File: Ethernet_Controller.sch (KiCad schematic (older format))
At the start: 31 parts, among them J1 5-2337992-8, U1 RTL8111H, Y1 ABM8G-25.000MHZ-18-D2Y-T

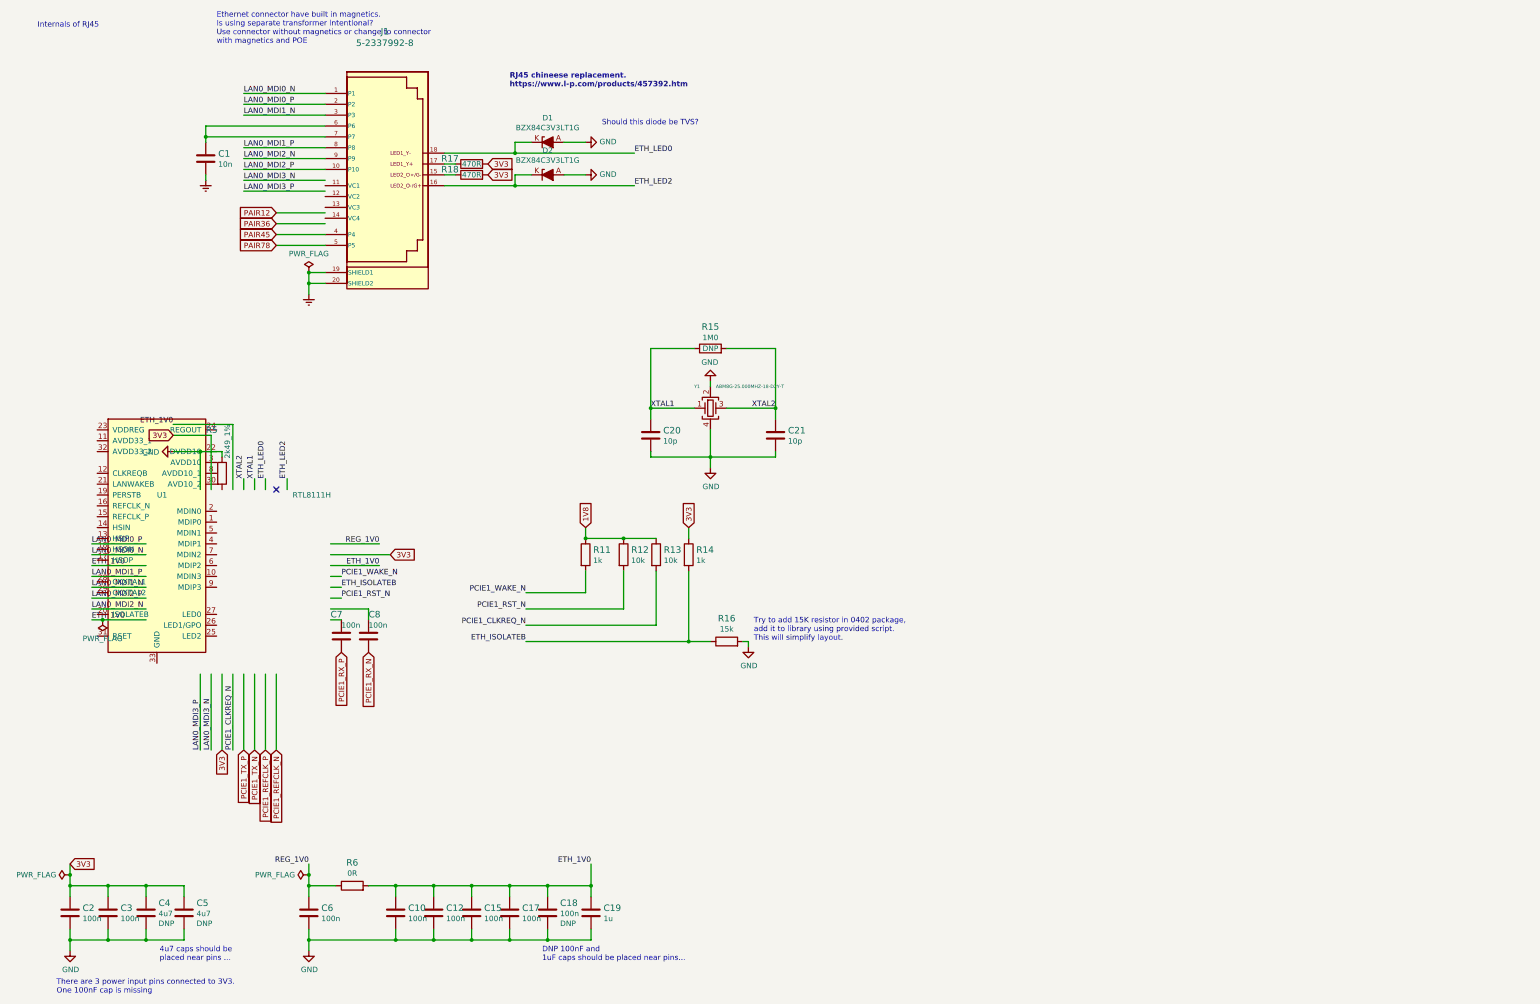
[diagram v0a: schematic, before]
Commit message: Cleanign Ethernet_Controller.sch
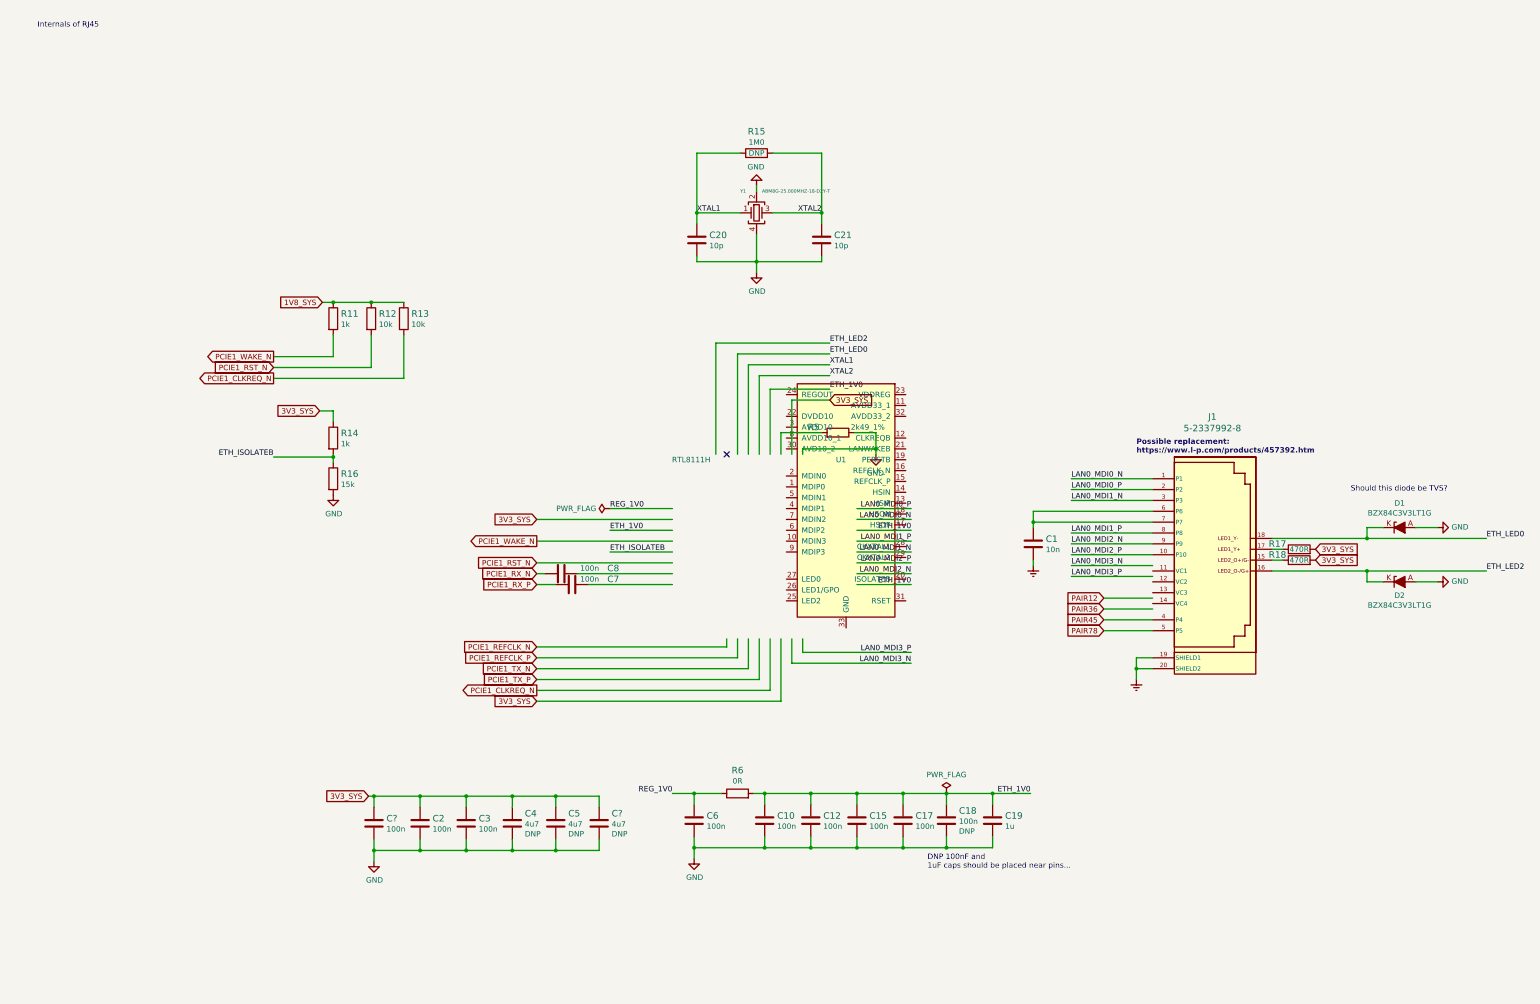
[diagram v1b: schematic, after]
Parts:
- added C?: C_100n_0402, sa800u-baseboard-hw-footprints:0402-cap, symbol sa800u-baseboard-hw:C_100n_0402
- added C?: C_4u7_0402, sa800u-baseboard-hw-footprints:0402-cap, symbol sa800u-baseboard-hw:C_4u7_0402
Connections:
- net labels added: 1V8_SYS, 3V3_SYS
- net labels removed: 1V8, 3V3
- wire segments 149 -> 169
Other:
- note added: "Possible replacement:\nhttps://www.l-p.com/products/457392.htm"
- note removed: "4u7 caps should be \nplaced near pins ..."
- note removed: "Ethernet connector have built in magnetics. \nIs using separate transformer intentional?\nUse connector without magnetics or change to connector \nwith magnetics and POE"
- note removed: "RJ45 chineese replacement. \nhttps://www.l-p.com/products/457392.htm"
- note removed: "There are 3 power input pins connected to 3V3.\nOne 100nF cap is missing"
- note removed: "Try to add 15K resistor in 0402 package,\nadd it to library using provided script.\nThis will simplify layout."
- moved on the sheet: C1, C10, C12, C15, C17, C18, C19, C2, C20, C21, C3, C4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
